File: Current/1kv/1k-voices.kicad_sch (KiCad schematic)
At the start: 152 parts, among them J2 Conn_01x05, J5 Qwiic, J6 JTAG, J7 ISP, J8 Reset, K0 Switch, K1 Switch, K10 Switch, K11 Switch, K12 Switch, K13 Switch, K14 Switch, K15 Switch, K16 Switch, K17 Switch, K18 Switch, K19 Switch, K2 Switch, K20 Switch, K21 Switch, K22 Switch, K23 Switch, K24 Switch, K25 Switch, K26 Switch, K27 Switch, K28 Switch, K29 Switch, K3 Switch, K30 Switch, K31 Switch, K32 Switch, K33 Switch, K34 Switch, K35 Switch, K36 Switch, K37 Switch, K38 Switch, K39 Switch, K4 Switch, K40 Switch, K41 Switch, K42 Switch, K43 Switch, K44 Switch, K45 Switch, K46 Switch, K47 Switch, K48 Switch, K49 Switch, K5 Switch, K50 Switch, K51 Switch, K52 Switch, K53 Switch, K54 Switch, K55 Switch, K56 Switch, K57 Switch, K58 Switch, K59 Switch, K6 Switch, K60 Switch, K61 Switch, K62 Switch, K63 Switch, K7 Switch, K8 Switch, K9 Switch, SW1 SW_DIP_x04, SW2 Rotary_Encoder, SW3 Rotary_Encoder, U1 ATMEGA32A-PU, U2 LD1117S33TR_SOT223, Y1 Crystal

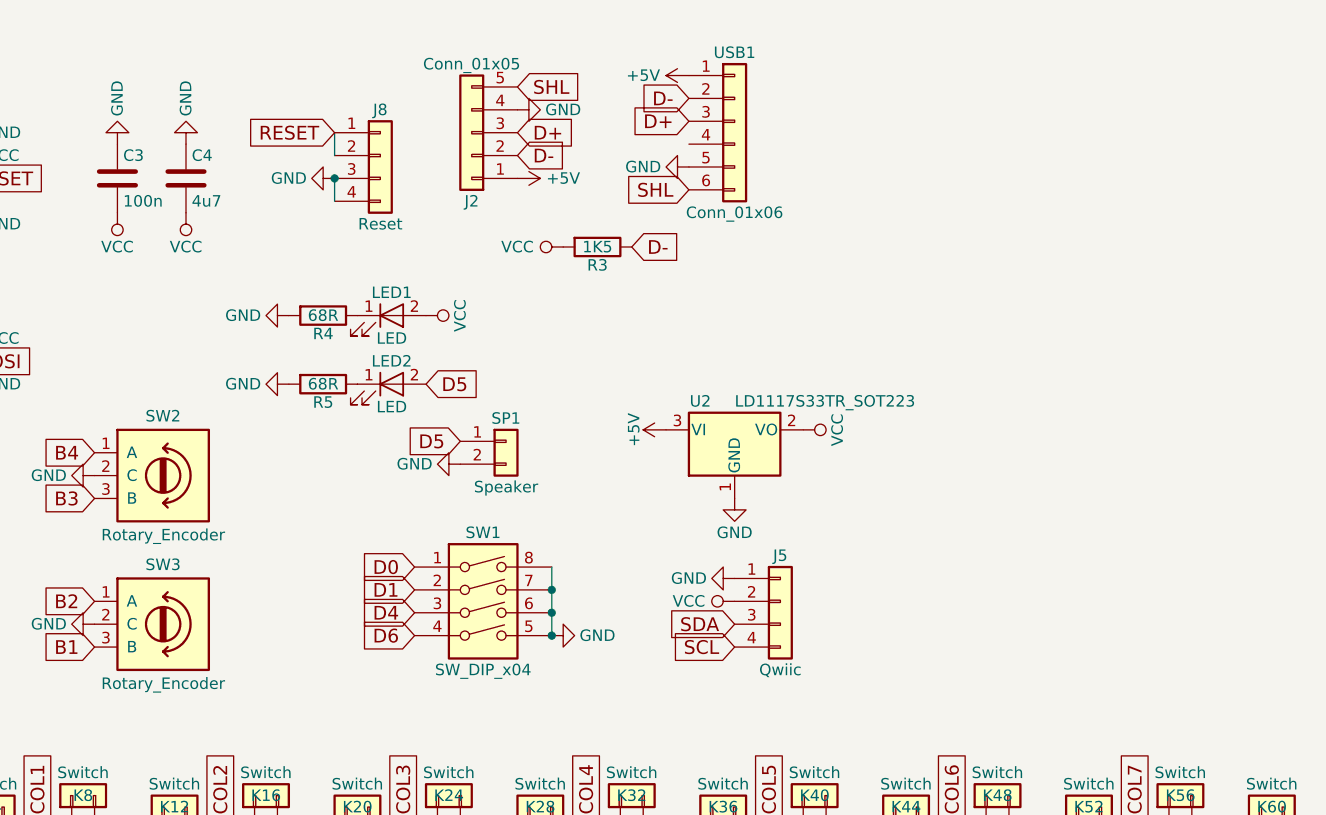
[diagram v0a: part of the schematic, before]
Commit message: QSS Upload
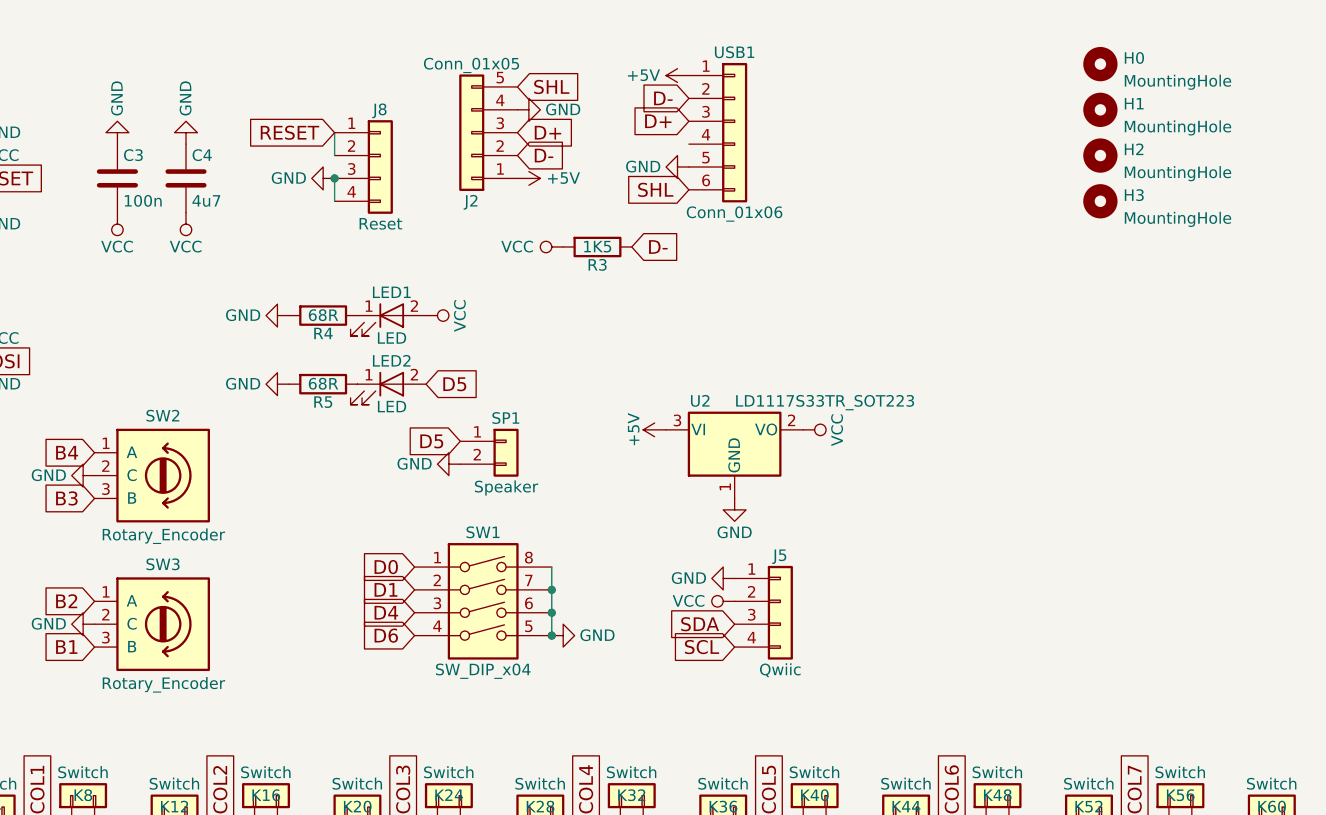
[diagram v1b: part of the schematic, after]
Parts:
- added H0, H1, H2, H3: MountingHole, MountingHole:MountingHole_3.2mm_M3, symbol Mechanical:MountingHole
- J5: footprint olkb:JST_SH_SM04B-SRSS-TB_04x1.00mm_Angled-SZ-combined -> Connector_PinHeader_2.54mm:PinHeader_1x04_P2.54mm_Vertical
